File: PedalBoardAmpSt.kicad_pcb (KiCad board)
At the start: 2 copper layers, 112.8 x 48.3 mm, 36 parts, among them J1 R-IN, J2 DC_IN, J3 out, J4 L-IN, J5 L-OUT, SW1 SDBY_MUTE, U1 TDA7293, U2 TDA7293

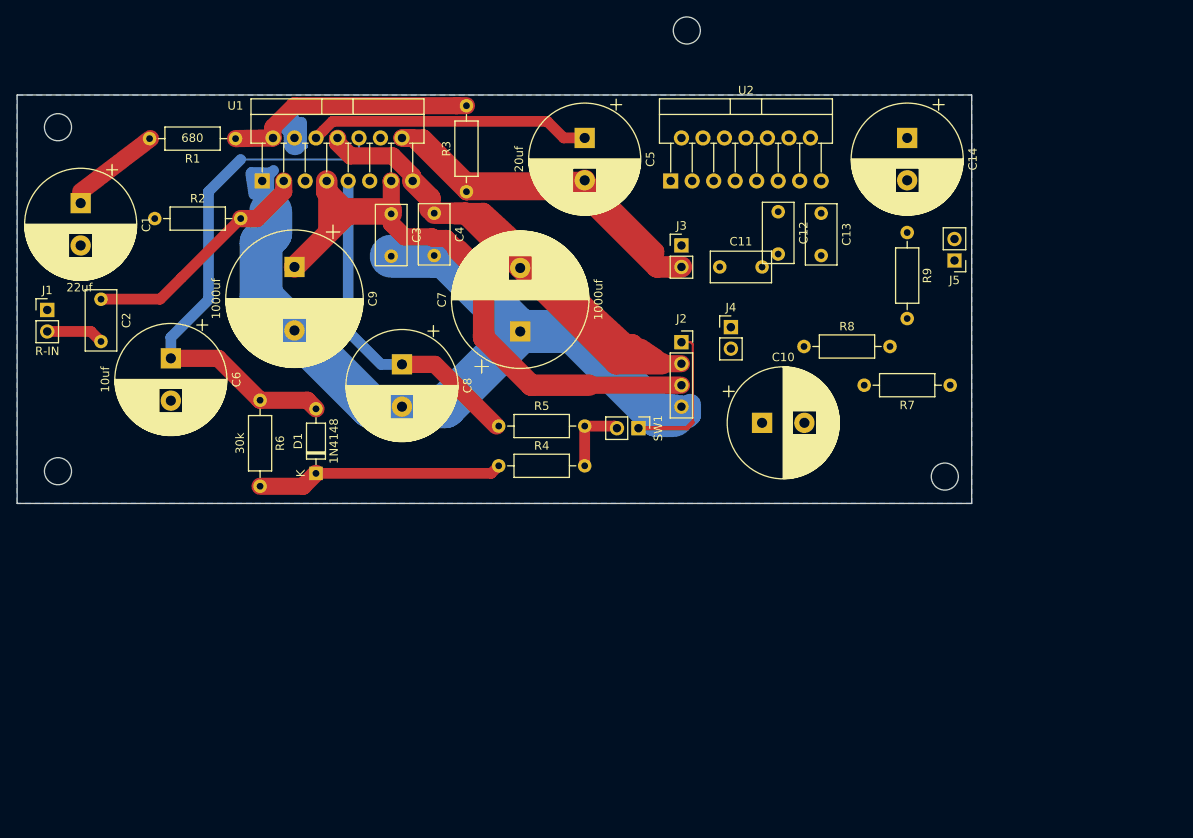
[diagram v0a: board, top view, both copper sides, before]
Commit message: re-layout
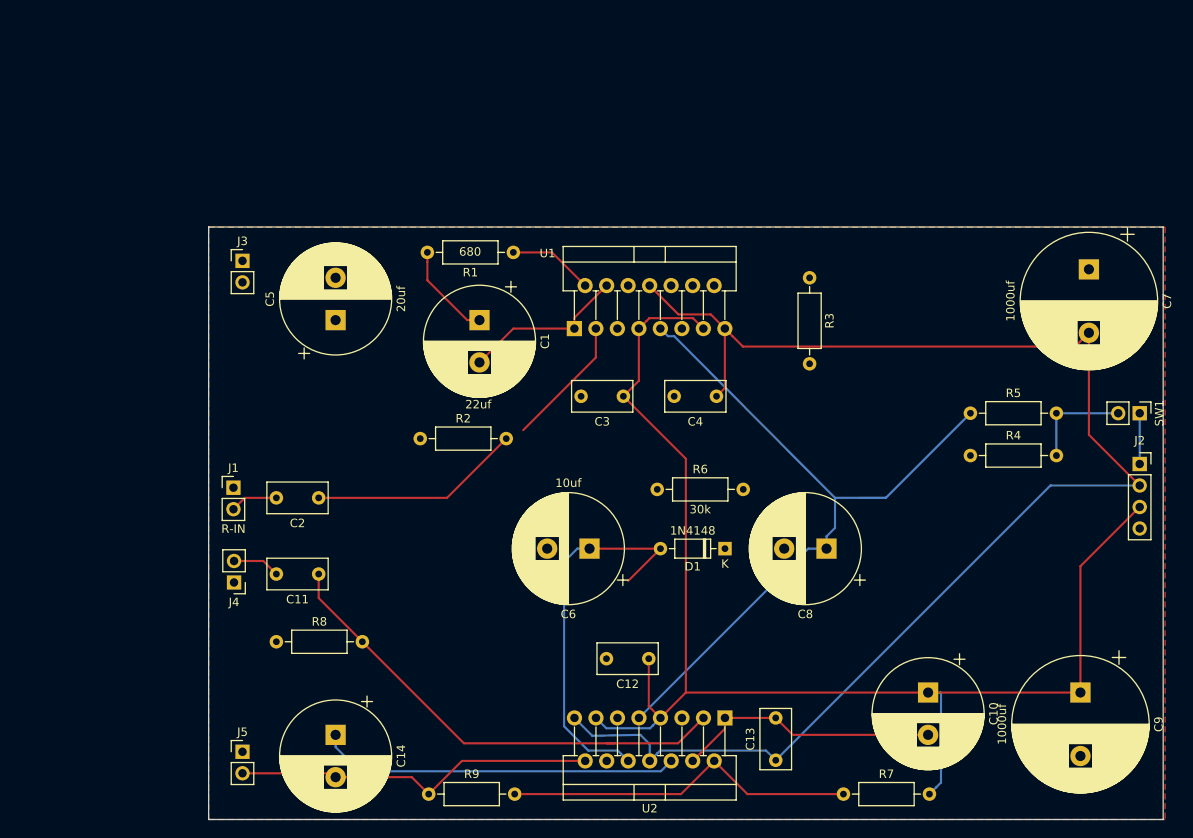
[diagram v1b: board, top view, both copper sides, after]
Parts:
- removed H1, H2, H3, H4: MountingHole, MountingHole:MountingHole_3.2mm_M3
- moved C9 105.6 mm to (197.0, 96.0)
- moved J5 102.2 mm to (98.0, 103.0), turned to 0 degrees
- moved C14 97.6 mm to (109.0, 101.0)
- moved R9 87.2 mm to (120.0, 108.0), turned to 0 degrees
- moved R8 71.4 mm to (102.0, 90.0)
- moved C7 67.6 mm to (198.0, 46.0), turned to 270 degrees
- moved J4 66.0 mm to (97.0, 83.0), turned to 180 degrees
- moved C13 64.9 mm to (161.0, 104.0), turned to 90 degrees
- moved U2 63.8 mm to (155.0, 99.0), turned to 180 degrees
- moved C11 59.7 mm to (107.0, 82.0), turned to 180 degrees
- moved SW1 59.2 mm to (204.0, 63.0)
- moved J2 56.0 mm to (204.0, 69.0)
- moved R5 55.8 mm to (184.0, 63.0)
- moved R4 55.7 mm to (184.0, 68.0)
- moved C12 55.0 mm to (146.0, 92.0), turned to 180 degrees
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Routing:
- net GND: track 152.0 -> 51.0 mm
- net -48vFilter: track 83.6 -> 169.0 mm
- net Net-(C5-Pad2): track 81.4 -> 0.00 mm
- net Net-(C11-Pad1): track 0.00 -> 57.7 mm
- net +48vFilter: track 94.3 -> 147.3 mm
- net STBY: track 39.9 -> 89.1 mm
- net Net-(C14-Pad2): track 0.00 -> 43.1 mm
- net Net-(C14-Pad1): track 0.00 -> 42.8 mm
- net Net-(R7-Pad1): track 0.00 -> 42.1 mm
- net Net-(C5-Pad1): track 33.4 -> 0.00 mm
- net Net-(D1-Pad1): track 29.2 -> 0.00 mm
- net Net-(R1-Pad1): track 29.6 -> 10.1 mm
- net MUTE: track 62.4 -> 46.5 mm
- net Net-(C10-Pad1): track 0.00 -> 14.0 mm
- net Net-(C2-Pad1): track 28.1 -> 40.6 mm
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- added copper zone on F.Cu, net GND
- removed copper zone on B.Cu, net GND
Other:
- board size 112.8 x 48.3 mm -> 112.8 x 70 mm

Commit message: larger traces
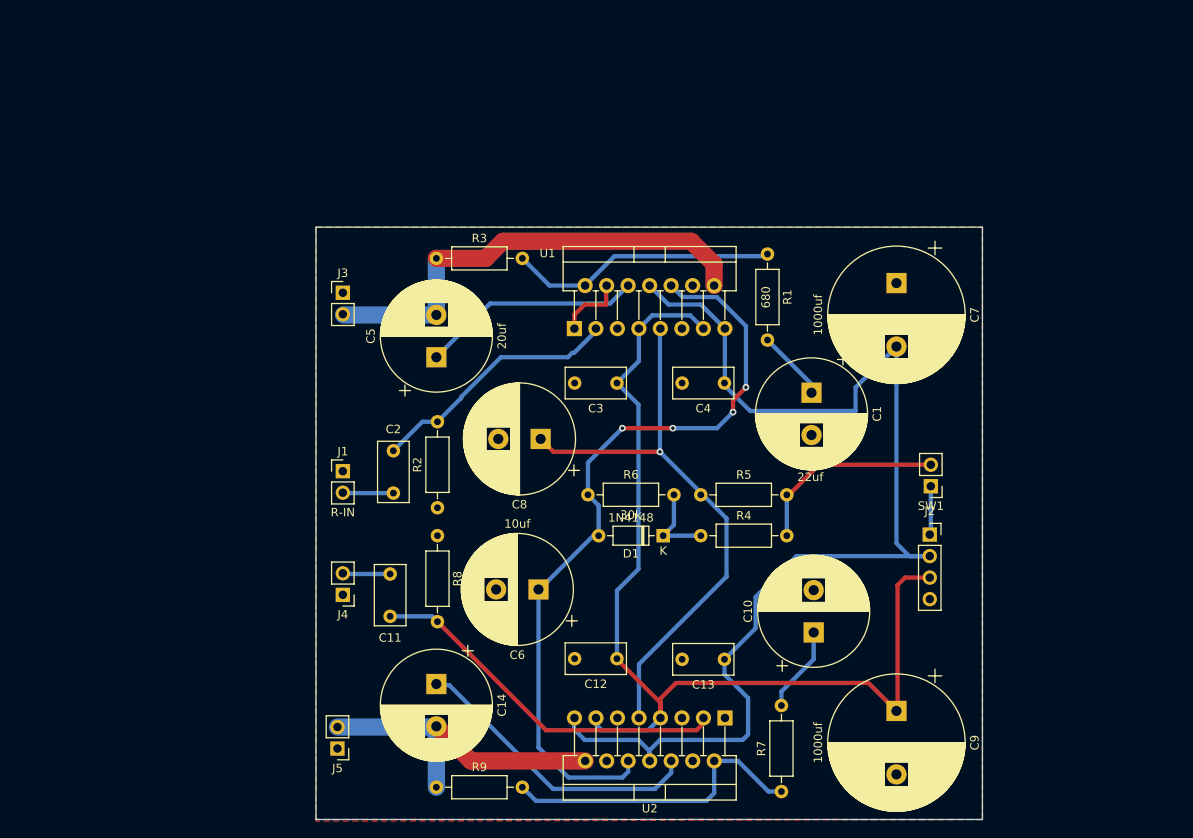
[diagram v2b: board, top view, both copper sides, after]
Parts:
- moved R3 44.2 mm to (120.9, 44.7), turned to 0 degrees
- moved C1 40.2 mm to (165.2, 60.6)
- moved C8 36.2 mm to (133.2, 66.0)
- moved R5 33.3 mm to (152.1, 72.6)
- moved R4 33.2 mm to (152.1, 77.5)
- moved R1 30.0 mm to (160.0, 44.2), turned to 270 degrees
- moved J2 26.2 mm to (179.2, 77.3)
- moved SW1 26.1 mm to (179.3, 71.6), turned to 180 degrees
- moved C7 22.8 mm to (175.3, 47.6)
- moved R8 22.8 mm to (121.0, 77.5), turned to 270 degrees
- moved C9 21.8 mm to (175.3, 98.2)
- moved C10 15.3 mm to (165.5, 88.9), turned to 90 degrees
- moved C13 13.4 mm to (154.9, 92.1), turned to 180 degrees
- moved C14 13.3 mm to (120.9, 95.0)
- moved J1 13.1 mm to (109.9, 69.8)
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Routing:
- net Net-(C5-Pad2): track 0.00 -> 55.1 mm
- net MUTE: track 46.5 -> 92.7 mm, vias 0 -> 5
- net GND: track 51.0 -> 8.15 mm
- net -48vFilter: track 169.0 -> 139.6 mm
- net +48vFilter: track 147.3 -> 120.9 mm
- net Net-(C5-Pad1): track 0.00 -> 26.2 mm
- net Net-(R1-Pad1): track 10.1 -> 31.1 mm
- net STBY: track 89.1 -> 68.4 mm, vias 0 -> 1
- net Net-(C11-Pad1): track 57.7 -> 43.6 mm
- net Net-(R4-Pad2): track 12.3 -> 23.1 mm
- net Net-(C2-Pad1): track 40.6 -> 30.2 mm
- net Net-(D1-Pad1): track 0.00 -> 9.81 mm
- net Net-(C14-Pad1): track 42.8 -> 35.3 mm
- net Net-(C14-Pad2): track 43.1 -> 37.9 mm
- net Net-(R7-Pad1): track 42.1 -> 37.0 mm
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- added copper zone on B.Cu, net GND
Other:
- board size 112.8 x 70 mm -> 78.7 x 70 mm

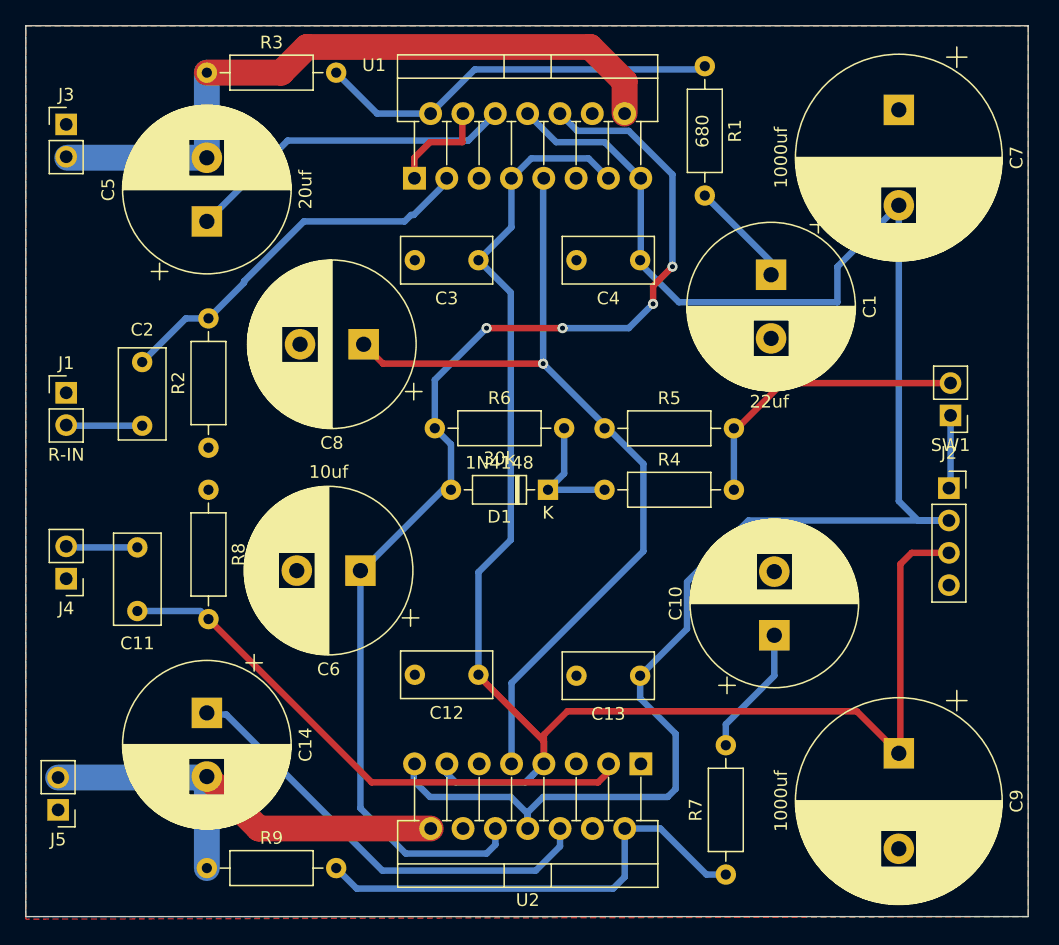
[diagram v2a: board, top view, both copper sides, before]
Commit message: update design
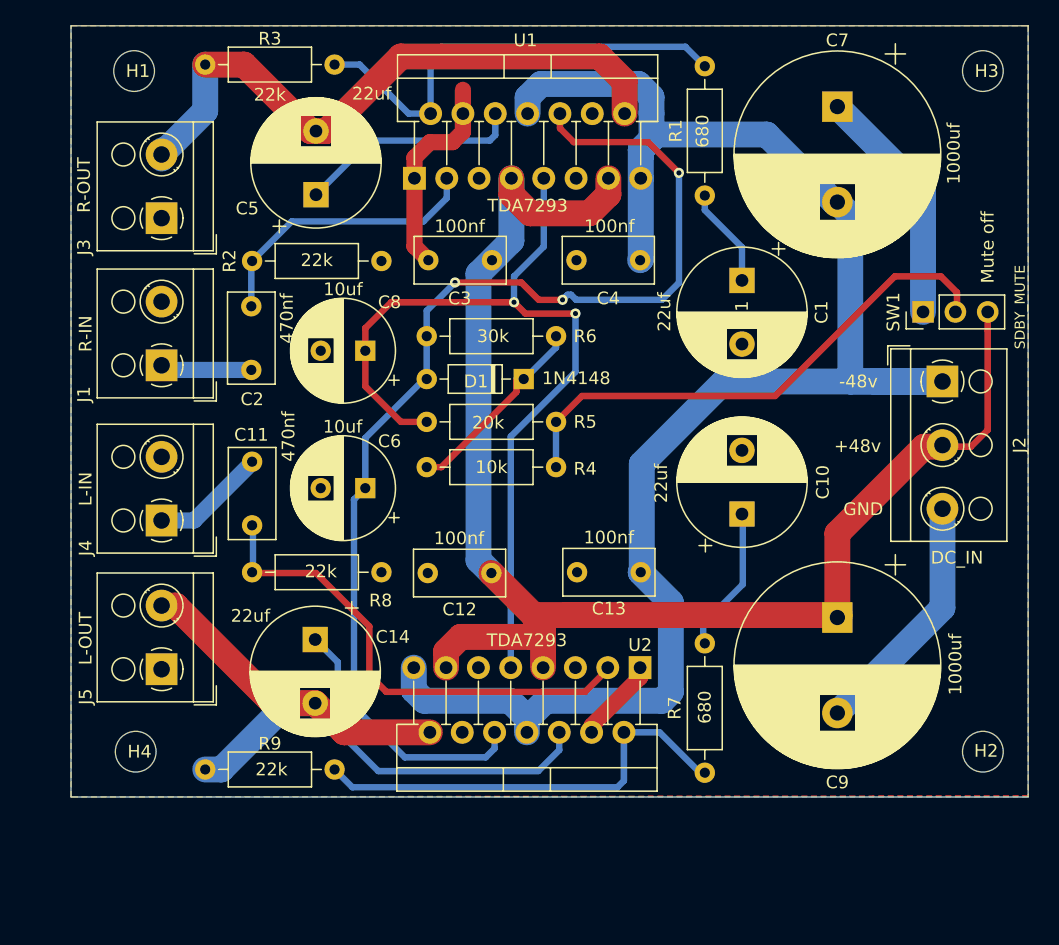
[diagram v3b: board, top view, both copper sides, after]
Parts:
- added H1: MountingHole, MountingHole:MountingHole_3.2mm_M3, F.Cu at (115.2, 44.6)
- added H2: MountingHole, MountingHole:MountingHole_3.2mm_M3, F.Cu at (181.9, 98.0)
- added H3: MountingHole, MountingHole:MountingHole_3.2mm_M3, F.Cu at (181.9, 44.6)
- added H4: MountingHole, MountingHole:MountingHole_3.2mm_M3, F.Cu at (115.3, 98.0)
- C1, C10: footprint Capacitor_THT:CP_Radial_D13.0mm_P5.00mm -> Capacitor_THT:CP_Radial_D10.0mm_P5.00mm
- C14, C5: value 20uf -> 22uf; footprint Capacitor_THT:CP_Radial_D13.0mm_P5.00mm -> Capacitor_THT:CP_Radial_D10.0mm_P5.00mm
- C6, C8: footprint Capacitor_THT:CP_Radial_D13.0mm_P5.00mm -> Capacitor_THT:CP_Radial_D8.0mm_P3.50mm
- J1, J4, J5: footprint Connector_PinHeader_2.54mm:PinHeader_1x02_P2.54mm_Vertical -> TerminalBlock_RND:TerminalBlock_RND_205-00001_1x02_P5.00mm_Horizontal
- J2: footprint Connector_PinSocket_2.54mm:PinSocket_1x04_P2.54mm_Vertical -> TerminalBlock_RND:TerminalBlock_RND_205-00002_1x03_P5.00mm_Horizontal
- J3: value out -> R-OUT; footprint Connector_PinHeader_2.54mm:PinHeader_1x02_P2.54mm_Vertical -> TerminalBlock_RND:TerminalBlock_RND_205-00001_1x02_P5.00mm_Horizontal
- SW1: footprint Connector_PinHeader_2.54mm:PinHeader_1x02_P2.54mm_Vertical -> Connector_PinHeader_2.54mm:PinHeader_1x03_P2.54mm_Vertical
- moved R2 20.0 mm to (134.6, 59.5), turned to 180 degrees
- moved R8 15.1 mm to (134.6, 83.9), turned to 180 degrees
- moved R4 14.1 mm to (138.2, 75.7)
- moved R5 14.0 mm to (138.2, 72.1)
- moved J5 13.7 mm to (117.3, 91.6), turned to 90 degrees
- moved C9 11.7 mm to (170.4, 87.5)
- moved C11 11.3 mm to (124.5, 80.3)
- moved J3 10.5 mm to (117.3, 56.1), turned to 90 degrees
- moved C14 10.3 mm to (129.4, 89.2)
- moved C10 9.86 mm to (162.9, 79.4)
- moved C2 9.63 mm to (124.4, 63.1)
- moved D1 8.91 mm to (145.8, 68.8)
- moved C5 8.82 mm to (129.5, 54.3)
- moved J4 8.78 mm to (117.3, 79.9), turned to 90 degrees
- moved SW1 8.41 mm to (177.2, 63.5), turned to 90 degrees
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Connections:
- J1 pad 1: GND -> Net-(C2-Pad2)
- J1 pad 2: Net-(C2-Pad2) -> GND
- J2 pad 1: +5V -> -48vFilter
- J2 pad 2: -48vFilter -> +48vFilter
- J2 pad 3: +48vFilter -> GND
- J4 pad 1: GND -> Net-(C11-Pad2)
- J4 pad 2: Net-(C11-Pad2) -> GND
- SW1 pad 1: +5V -> GND
- U1 pad 11: Net-(U1-Pad11) -> (no net)
- U1 pad 12: Net-(U1-Pad12) -> (no net)
- U1 pad 5: Net-(U1-Pad5) -> (no net)
- U2 pad 11: Net-(U2-Pad11) -> (no net)
- U2 pad 12: Net-(U2-Pad12) -> (no net)
- U2 pad 5: Net-(U2-Pad5) -> (no net)
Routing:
- net GND: track 8.15 -> 61.5 mm
- net Net-(R4-Pad2): track 23.1 -> 41.8 mm
- net Net-(C5-Pad1): track 26.2 -> 17.7 mm
- net Net-(C2-Pad1): track 30.2 -> 22.5 mm
- net Net-(C14-Pad1): track 35.3 -> 28.7 mm
- net +5V: track 5.77 -> 0.00 mm
- net Net-(D1-Pad1): track 9.81 -> 15.5 mm
- net Net-(C5-Pad2): track 55.1 -> 50.0 mm
- net Net-(C11-Pad1): track 43.6 -> 38.6 mm
- net Net-(R1-Pad1): track 31.1 -> 36.1 mm
- net Net-(C11-Pad2): track 5.62 -> 9.09 mm
- net Net-(C14-Pad2): track 37.9 -> 35.9 mm
- net Net-(R7-Pad1): track 37.0 -> 35.1 mm
- net MUTE: track 92.7 -> 90.9 mm, vias 5 -> 3
- net Net-(C10-Pad1): track 10.2 -> 11.8 mm
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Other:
- board size 78.7 x 70 mm -> 75.2 x 60.6 mm
- rule pad_to_mask_clearance: 0.051 -> 0
- board text added: "+48v"
- board text added: "-48v"
- board text added: "GND"
- board text added: "Mute off"
